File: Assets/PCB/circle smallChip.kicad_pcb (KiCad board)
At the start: 2 copper layers, 40.6 x 40.6 mm, 21 parts, among them j1 R_0805_2012Metric, j10 R_0805_2012Metric, j11 R_0805_2012Metric, j12 R_0805_2012Metric, j13 R_0805_2012Metric, j14 R_0805_2012Metric, j15 R_0805_2012Metric, j2 R_0805_2012Metric, j3 R_0805_2012Metric, j4 R_0805_2012Metric, j5 R_0805_2012Metric, j6 R_0805_2012Metric, j7 R_0805_2012Metric, j8 R_0805_2012Metric, j9 R_0805_2012Metric

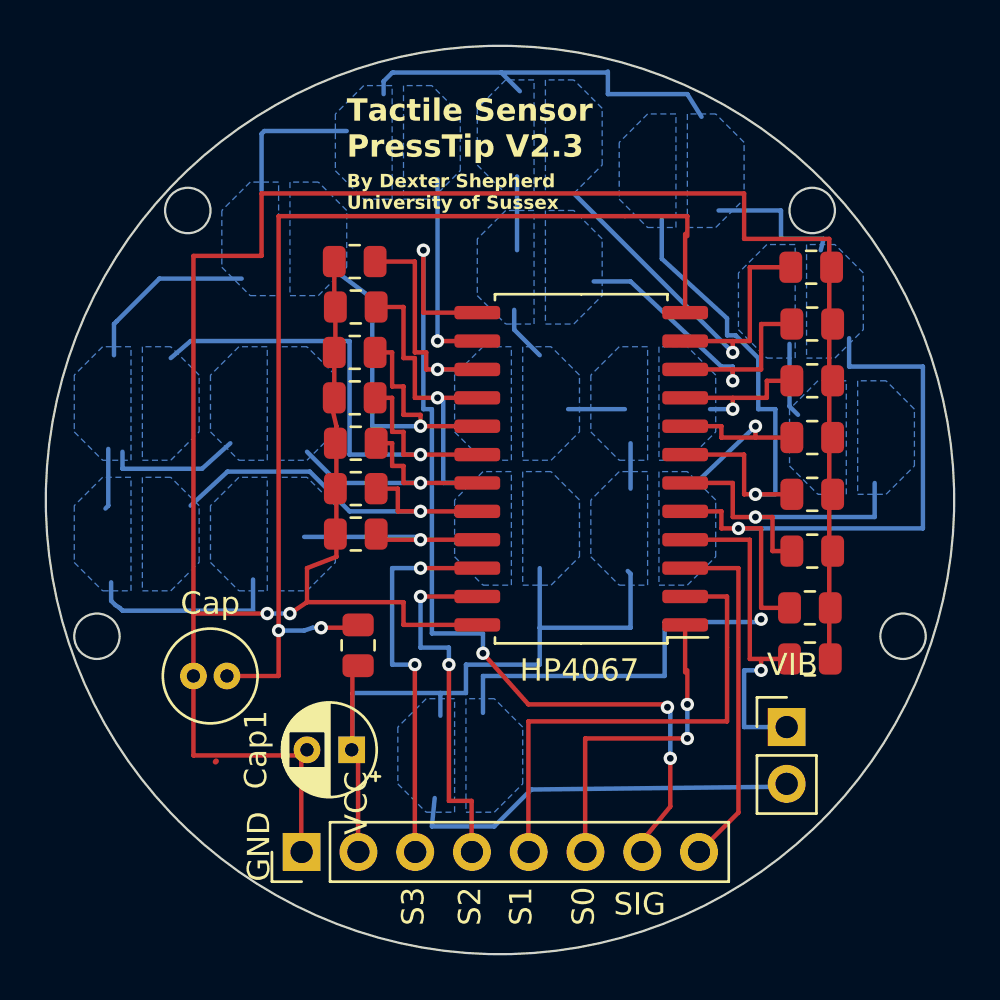
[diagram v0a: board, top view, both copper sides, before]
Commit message: updates to file
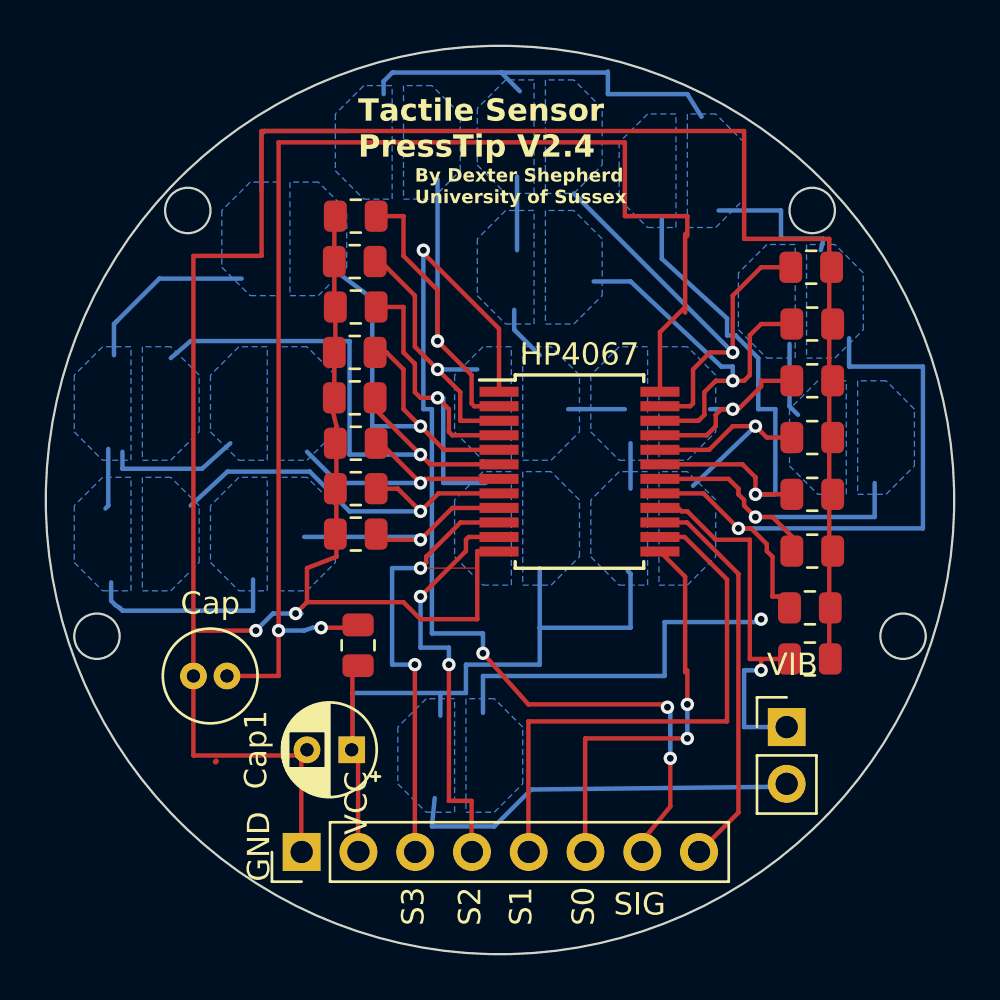
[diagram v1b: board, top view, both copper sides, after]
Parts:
- added j4.1: R_0805_2012Metric, Resistor_SMD:R_0805_2012Metric, F.Cu at (120.5, 89.2)
- HP4067: value SOIC-24W_7.5x15.4mm_P1.27mm -> SSOP-24_5.3x8.2mm_P0.65mm; footprint Package_SO:SOIC-24W_7.5x15.4mm_P1.27mm -> Package_SO:SSOP-24_5.3x8.2mm_P0.65mm
- moved HP4067 0.15 mm to (130.6, 100.6), turned to 0 degrees
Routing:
- net (no net): track 97.7 -> 252.7 mm
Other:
- board text added: "Tactile Sensor PressTip V2.4"
- board text removed: "Tactile Sensor PressTip V2.3"
